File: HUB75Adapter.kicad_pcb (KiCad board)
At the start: 2 copper layers, 100 x 93 mm, 41 parts, among them J1 Power input, J10 P1_SELECT_PIN4, J11 P1_SELECT_PIN8, J2 Power input, J3 I2C Extension, J4 Panel power 1, J5 Panel power 2, J6 Panel 1, J7 Panel 2, J8 P0_SELECT_PIN4, J9 P0_SELECT_PIN8, Q1 AOD403, U1 RaspberryPi Zero W, U2 74HCT245, U3 74HCT245, U4 74HCT245

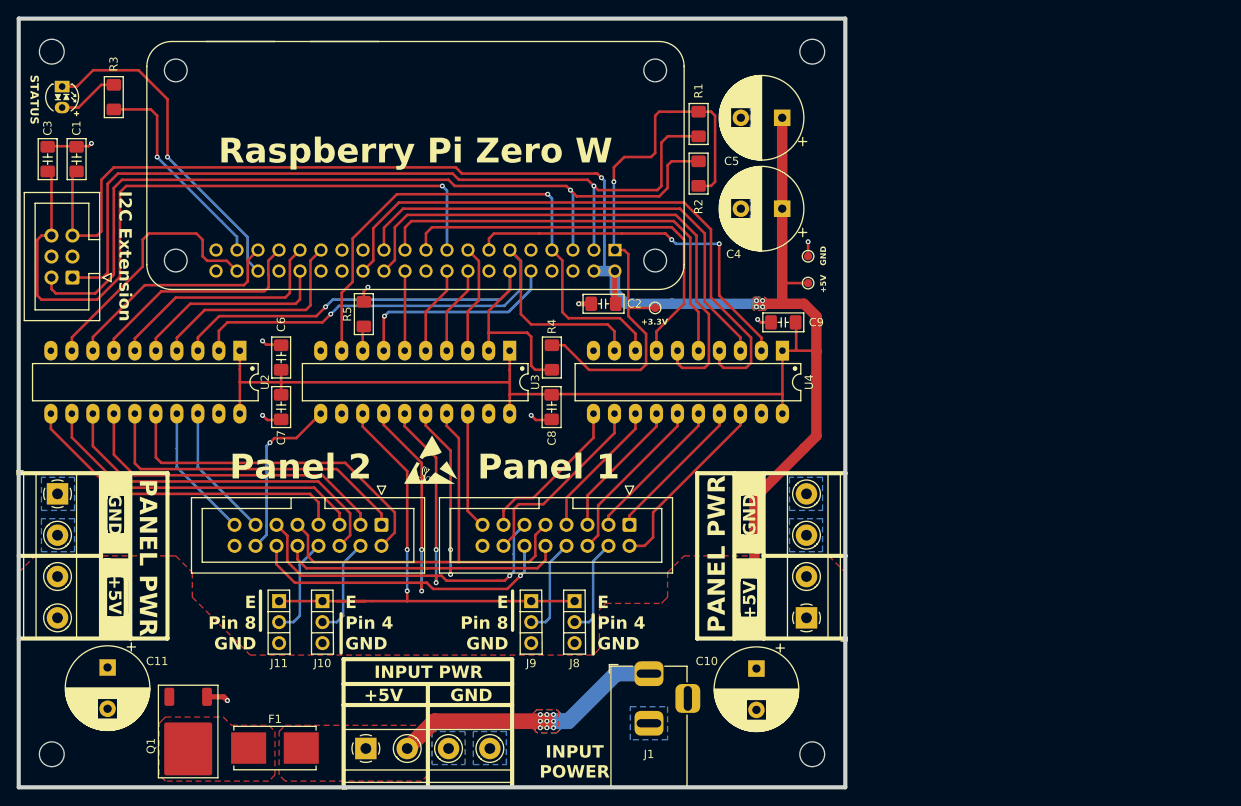
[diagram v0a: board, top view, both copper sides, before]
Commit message: Added plots and BOM
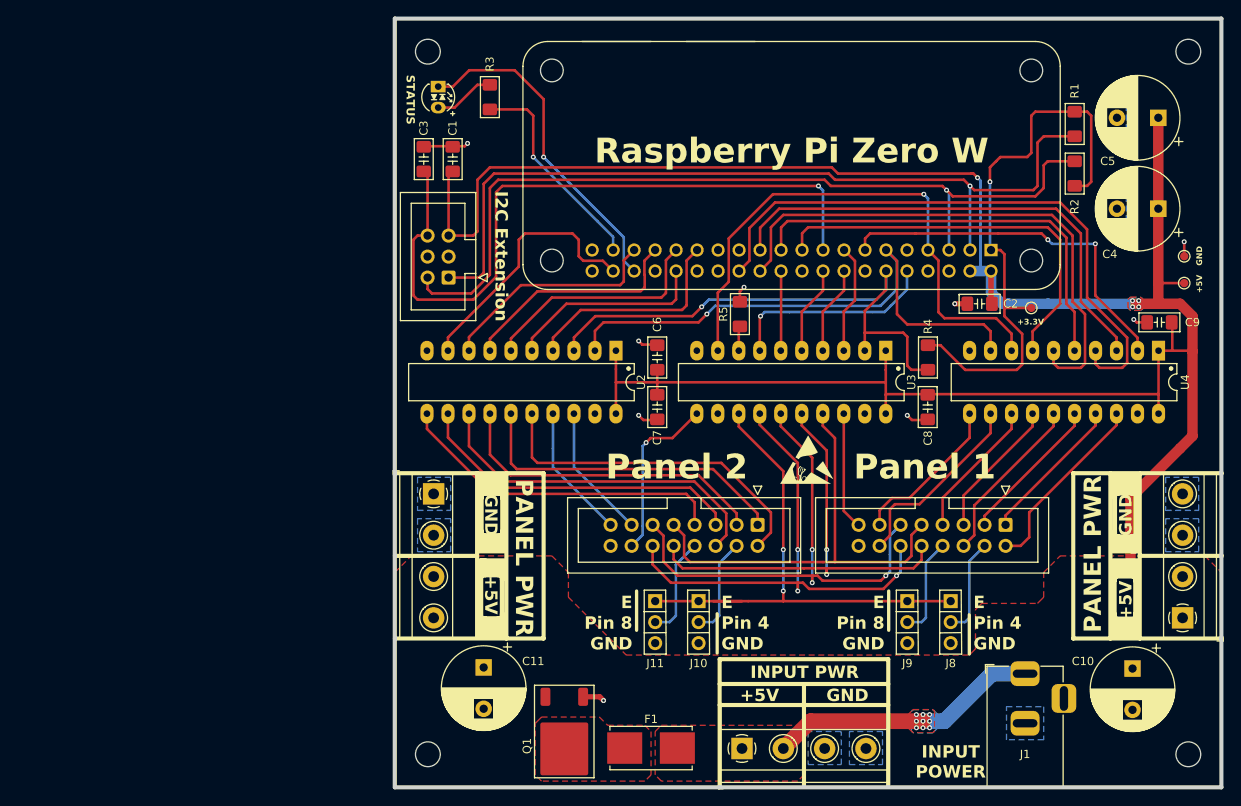
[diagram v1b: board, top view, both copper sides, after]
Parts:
- moved U3 45.5 mm to (154.9, 90.2)
- moved C1 45.5 mm to (102.5, 67.0)
- moved C10 45.5 mm to (184.8, 128.6)
- moved C11 45.5 mm to (106.2, 128.5)
- moved C2 45.5 mm to (166.2, 84.5)
- moved C3 45.5 mm to (99.0, 67.0)
- moved C4 45.5 mm to (187.9, 73.0)
- moved C5 45.5 mm to (187.9, 62.0)
- moved C6 45.5 mm to (127.2, 91.0)
- moved C7 45.5 mm to (127.2, 97.0)
- moved C8 45.5 mm to (160.0, 97.0)
- moved C9 45.5 mm to (188.0, 86.8)
- moved F1 45.5 mm to (126.5, 138.2)
- moved G*** 45.5 mm to (145.5, 103.5)
- moved G*** 45.5 mm to (134.0, 66.0)
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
